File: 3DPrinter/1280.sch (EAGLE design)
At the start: 71 parts, among them IC1 ATMEGA1280-16AU, IC2 7805DT, IC3 CP2102, IC4 X, IC5 Y, IC6 Z, IC7 E0, IC8 E1, Q1 16 MHz, X1 PN61729-S, X11 CON-CP-03, X12 CON-CP-03, X13 CON-CP-03, X14 CON-CP-03, X15 CON-CP-03, X16 CON-CP-03, X2 CON-5.08-03P, X3 CON-5.08-03P, X4 CON-7.62-02P, X5 CON-CP-04, X6 CON-CP-04, X7 CON-CP-04, X8 CON-CP-04, X9 CON-CP-04

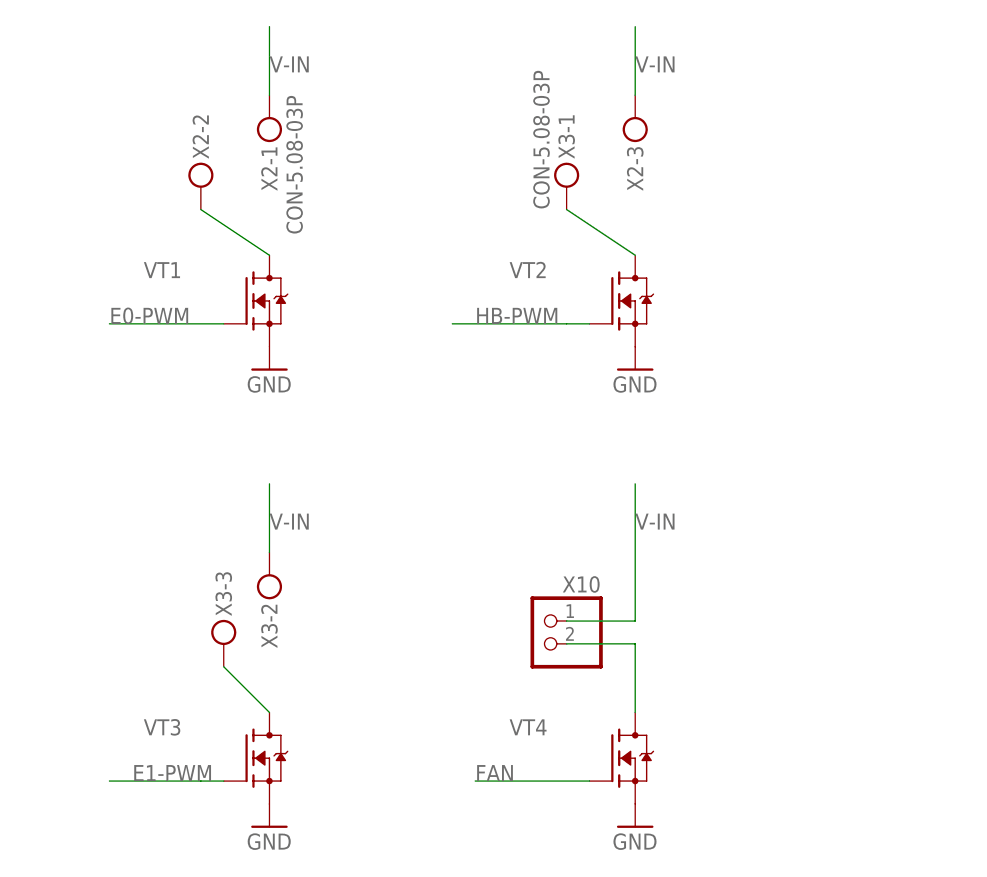
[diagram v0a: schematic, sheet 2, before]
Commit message: _
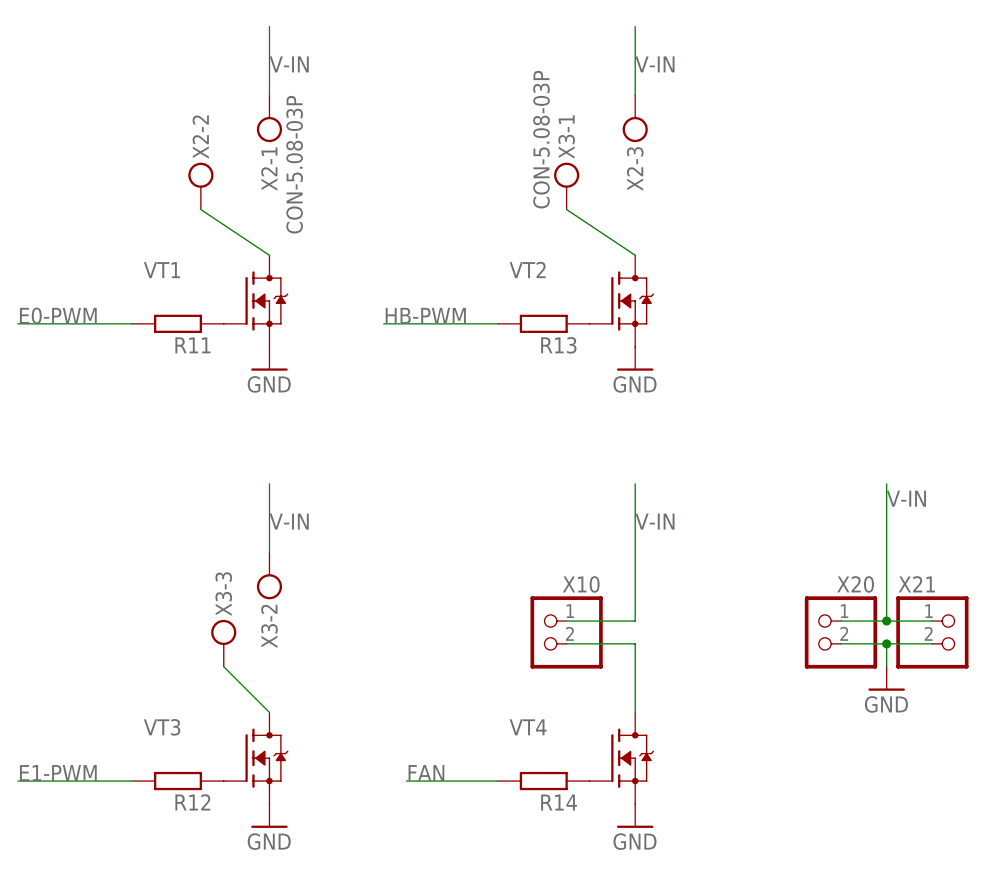
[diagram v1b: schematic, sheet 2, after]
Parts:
- added R11, R12, R13, R14: (no value), Namenlos:R_0805
- added X20, X21: (no value), Namenlos:CON-CP-02
- JP1: device avr-7:AVR-ISP-6VERT -> pinhead:PINHD-2X3
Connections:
- new net N$44: R11.1, VT1.G
- new net N$45: R13.1, VT2.G
- new net N$46: R14.1, VT4.G
- new net N$47: R12.1, VT3.G
- net E0-PWM: now also R11.2; no longer VT1.G
- net E1-PWM: now also R12.2; no longer VT3.G
- net FAN: now also R14.2; no longer VT4.G
- net GND: now also X20.2, X21.2
- net HB-PWM: now also R13.2; no longer VT2.G
- net V-IN: now also X20.1, X21.1
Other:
- note added: "MISO"
- note added: "MOSI"
- note added: "RST"
- note added: "SCK"
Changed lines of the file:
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@@
 <part name="P+1" library="supply1" deviceset="+5V" device=""/>
 <part name="R1" library="Namenlos" deviceset="R_" device="0805" value="20k"/>
-<part name="JP1" library="avr-7" deviceset="AVR-ISP-6" device="VERT" value="AVR-ISP-6VERT"/>
+<part name="JP1" library="pinhead" deviceset="PINHD-2X3" device="" value="AVR-ISP-6VERT"/>
 <part name="P+2" library="supply1" deviceset="+5V" device=""/>
 <part name="GND3" library="supply1" deviceset="GND" device=""/>
@@
 <part name="S5" library="Namenlos" deviceset="SW-DIP03S" device=""/>
 <part name="P+26" library="supply1" deviceset="+5V" device=""/>
+<part name="R11" library="Namenlos" deviceset="R_" device="0805"/>
+<part name="R12" library="Namenlos" deviceset="R_" device="0805"/>
+<part name="R13" library="Namenlos" deviceset="R_" device="0805"/>
+<part name="R14" library="Namenlos" deviceset="R_" device="0805"/>
+<part name="X20" library="Namenlos" deviceset="CON-CP-02" device=""/>
+<part name="X21" library="Namenlos" deviceset="CON-CP-02" device=""/>
+<part name="GND36" library="supply1" deviceset="GND" device=""/>
 </parts>
 <sheets>
@@
 <instance part="X3" gate="-3" x="30.48" y="35.56" rot="MR90"/>
 <instance part="X10" gate="X$1" x="66.04" y="35.56" rot="MR0"/>
+<instance part="R11" gate="G$1" x="25.4" y="71.12" rot="R180"/>
+<instance part="R12" gate="G$1" x="25.4" y="20.32" rot="R180"/>
+<instance part="R13" gate="G$1" x="66.04" y="71.12" rot="R180"/>
+<instance part="R14" gate="G$1" x="66.04" y="20.32" rot="R180"/>
+<instance part="X20" gate="X$1" x="96.52" y="35.56" rot="MR0"/>
+<instance part="X21" gate="X$1" x="111.76" y="35.56"/>
+<instance part="GND36" gate="1" x="104.14" y="30.48"/>
 </instances>
 <busses>
@@
 <net name="E0-PWM" class="0">
 <segment>
-<pinref part="VT1" gate="G$1" pin="G"/>
-<wire x1="30.48" y1="71.12" x2="17.78" y2="71.12" width="0.1524" layer="91"/>
-<label x="17.78" y="71.12" size="1.778" layer="95"/>
+<label x="7.62" y="71.12" size="1.778" layer="95"/>
+<pinref part="R11" gate="G$1" pin="2"/>
+<wire x1="20.32" y1="71.12" x2="7.62" y2="71.12" width="0.1524" layer="91"/>
 </segment>
 </net>
 <net name="E1-PWM" class="0">
 <segment>
-<wire x1="27.94" y1="20.32" x2="17.78" y2="20.32" width="0.1524" layer="91"/>
-<pinref part="VT3" gate="G$1" pin="G"/>
-<wire x1="27.94" y1="20.32" x2="30.48" y2="20.32" width="0.1524" layer="91"/>
-<label x="20.32" y="20.32" size="1.778" layer="95"/>
+<wire x1="20.32" y1="20.32" x2="7.62" y2="20.32" width="0.1524" layer="91"/>
+<label x="7.62" y="20.32" size="1.778" layer="95"/>
+<pinref part="R12" gate="G$1" pin="2"/>
 </segment>
 </net>
 <net name="HB-PWM" class="0">
 <segment>
-<wire x1="68.58" y1="71.12" x2="55.88" y2="71.12" width="0.1524" layer="91"/>
-<label x="58.42" y="71.12" size="1.778" layer="95"/>
-<pinref part="VT2" gate="G$1" pin="G"/>
-<wire x1="68.58" y1="71.12" x2="71.12" y2="71.12" width="0.1524" layer="91"/>
+<label x="48.26" y="71.12" size="1.778" layer="95"/>
+<wire x1="60.96" y1="71.12" x2="48.26" y2="71.12" width="0.1524" layer="91"/>
+<pinref part="R13" gate="G$1" pin="2"/>
 </segment>
 </net>
 <net name="FAN" class="0">
 <segment>
-<pinref part="VT4" gate="G$1" pin="G"/>
-<wire x1="71.12" y1="20.32" x2="58.42" y2="20.32" width="0.1524" layer="91"/>
-<label x="58.42" y="20.32" size="1.778" layer="95"/>
+<label x="50.8" y="20.32" size="1.778" layer="95"/>
+<pinref part="R14" gate="G$1" pin="2"/>
+<wire x1="60.96" y1="20.32" x2="50.8" y2="20.32" width="0.1524" layer="91"/>
 </segment>
 </net>
@@
 <pinref part="VT1" gate="G$1" pin="S"/>
 <pinref part="GND9" gate="1" pin="GND"/>
+</segment>
+<segment>
+<pinref part="GND36" gate="1" pin="GND"/>
+<pinref part="X20" gate="X$1" pin="2"/>
+<wire x1="104.14" y1="33.02" x2="104.14" y2="35.56" width="0.1524" layer="91"/>
+<wire x1="104.14" y1="35.56" x2="99.06" y2="35.56" width="0.1524" layer="91"/>
+<pinref part="X21" gate="X$1" pin="2"/>
+<wire x1="109.22" y1="35.56" x2="104.14" y2="35.56" width="0.1524" layer="91"/>
+<junction x="104.14" y="35.56"/>
 </segment>
 </net>
@@
 <pinref part="X10" gate="X$1" pin="1"/>
 </segment>
+<segment>
+<wire x1="99.06" y1="38.1" x2="104.14" y2="38.1" width="0.1524" layer="91"/>
+<pinref part="X20" gate="X$1" pin="1"/>
+<pinref part="X21" gate="X$1" pin="1"/>
+<wire x1="104.14" y1="38.1" x2="109.22" y2="38.1" width="0.1524" layer="91"/>
+<wire x1="104.14" y1="38.1" x2="104.14" y2="53.34" width="0.1524" layer="91"/>
+<junction x="104.14" y="38.1"/>
+<label x="104.14" y="50.8" size="1.778" layer="95"/>
+</segment>
 </net>
 <net name="FAN-" class="0">
@@
 </segment>
 </net>
+<net name="N$44" class="0">
+<segment>
+<pinref part="VT1" gate="G$1" pin="G"/>
+<pinref part="R11" gate="G$1" pin="1"/>
+</segment>
+</net>
+<net name="N$45" class="0">
+<segment>
+<pinref part="VT2" gate="G$1" pin="G"/>
+<pinref part="R13" gate="G$1" pin="1"/>
+</segment>
+</net>
+<net name="N$46" class="0">
+<segment>
+<pinref part="VT4" gate="G$1" pin="G"/>
+<pinref part="R14" gate="G$1" pin="1"/>
+</segment>
+</net>
+<net name="N$47" class="0">
+<segment>
+<pinref part="VT3" gate="G$1" pin="G"/>
+<pinref part="R12" gate="G$1" pin="1"/>
+</segment>
+</net>
 </nets>
 </sheet>
 <sheet>
 <plain>
+<text x="40.64" y="165.1" size="1.778" layer="97">MISO</text>
+<text x="40.64" y="162.56" size="1.778" layer="97">SCK</text>
+<text x="40.64" y="160.02" size="1.778" layer="97">RST</text>
+<text x="60.96" y="162.56" size="1.778" layer="97">MOSI</text>
 </plain>
 <instances>
@@
 <instance part="P+1" gate="1" x="-22.86" y="127"/>
 <instance part="R1" gate="G$1" x="-15.24" y="114.3"/>
-<instance part="JP1" gate="G$1" x="53.34" y="162.56"/>
+<instance part="JP1" gate="A" x="53.34" y="162.56"/>
 <instance part="P+2" gate="1" x="66.04" y="170.18"/>
 <instance part="GND3" gate="1" x="66.04" y="154.94"/>
@@
 <segment>
 <wire x1="58.42" y1="162.56" x2="71.12" y2="162.56" width="0.1524" layer="91"/>
-<pinref part="JP1" gate="G$1" pin="4"/>
+<pinref part="JP1" gate="A" pin="4"/>
 </segment>
 <segment>
@@
 </segment>
 <segment>
-<wire x1="35.56" y1="162.56" x2="48.26" y2="162.56" width="0.1524" layer="91"/>
-<pinref part="JP1" gate="G$1" pin="3"/>
+<wire x1="35.56" y1="162.56" x2="50.8" y2="162.56" width="0.1524" layer="91"/>
+<pinref part="JP1" gate="A" pin="3"/>
 </segment>
 <segment>
@@
 </segment>
 <segment>
-<wire x1="35.56" y1="165.1" x2="48.26" y2="165.1" width="0.1524" layer="91"/>
-<pinref part="JP1" gate="G$1" pin="1"/>
+<wire x1="35.56" y1="165.1" x2="50.8" y2="165.1" width="0.1524" layer="91"/>
+<pinref part="JP1" gate="A" pin="1"/>
 </segment>
 <segment>
@@
 <wire x1="66.04" y1="157.48" x2="66.04" y2="160.02" width="0.1524" layer="91"/>
 <wire x1="66.04" y1="160.02" x2="58.42" y2="160.02" width="0.1524" layer="91"/>
-<pinref part="JP1" gate="G$1" pin="6"/>
+<pinref part="JP1" gate="A" pin="6"/>
 </segment>
 <segment>
@@
 <wire x1="66.04" y1="167.64" x2="66.04" y2="165.1" width="0.1524" layer="91"/>
 <wire x1="66.04" y1="165.1" x2="58.42" y2="165.1" width="0.1524" layer="91"/>
-<pinref part="JP1" gate="G$1" pin="2"/>
+<pinref part="JP1" gate="A" pin="2"/>
 </segment>
 <segment>
@@
 </segment>
 <segment>
-<wire x1="35.56" y1="160.02" x2="48.26" y2="160.02" width="0.1524" layer="91"/>
-<pinref part="JP1" gate="G$1" pin="5"/>
-</segment>
-<segment>
+<wire x1="35.56" y1="160.02" x2="50.8" y2="160.02" width="0.1524" layer="91"/>
+<pinref part="JP1" gate="A" pin="5"/>
+</segment>
+<segment>
